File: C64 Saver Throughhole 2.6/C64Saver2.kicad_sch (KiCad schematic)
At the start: 24 parts, among them J1 Conn_01x04, J2 Conn_01x08, J4 Conn_01x08, J5 Conn_01x04, J6 Conn_01x04, Q1 BC547, Q2 IRFR5305, U1 TL431LP

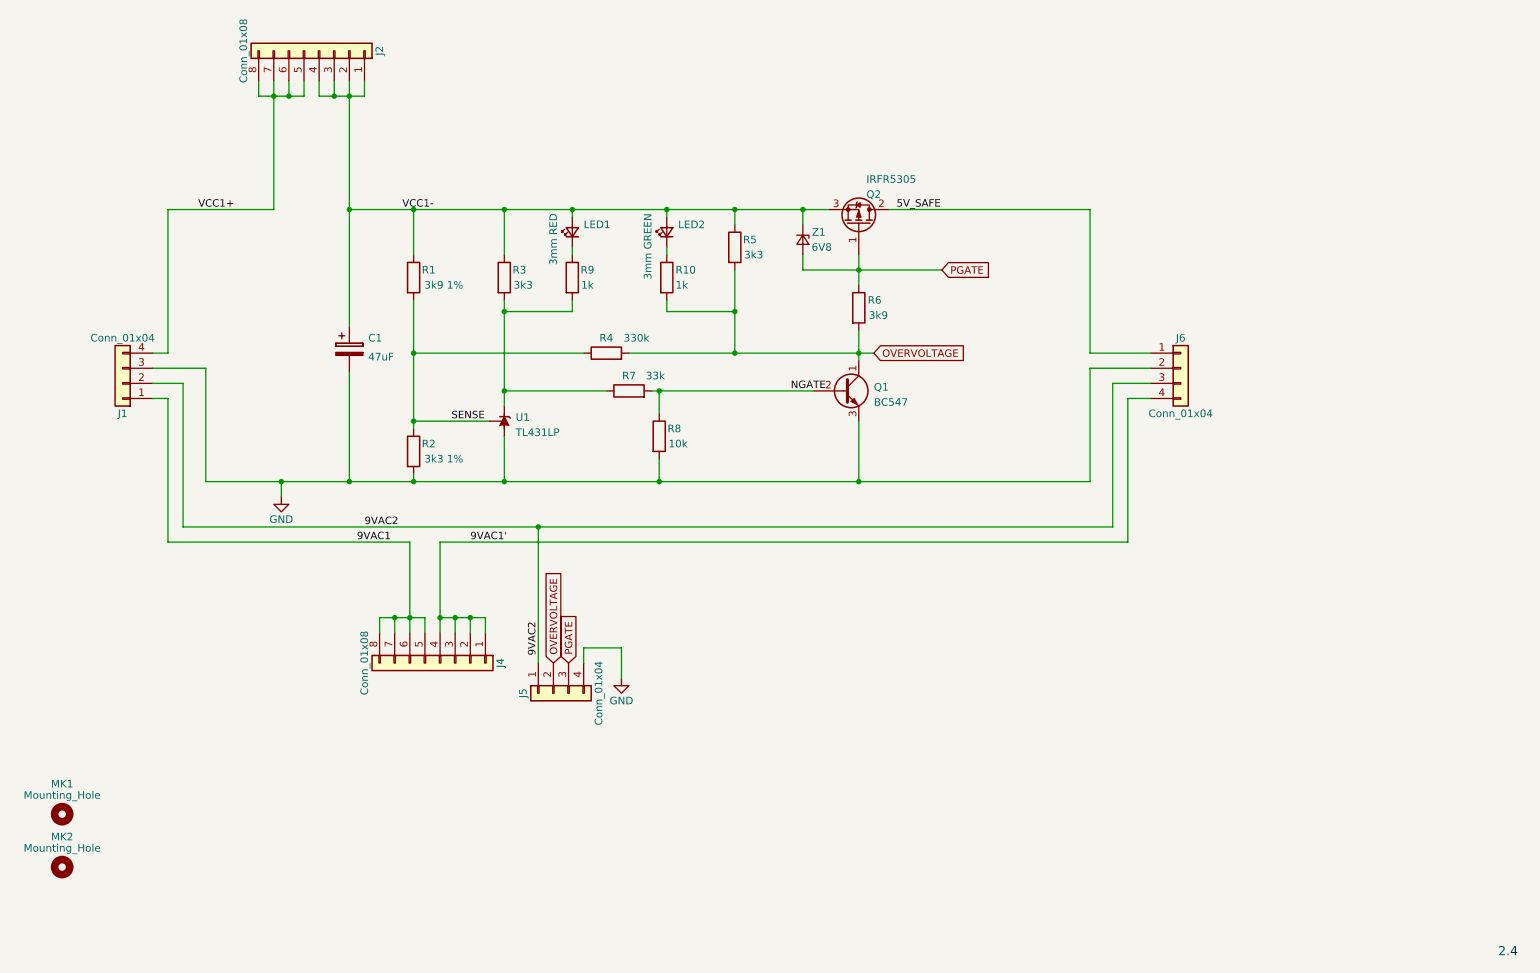
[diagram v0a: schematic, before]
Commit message: Preparing for Saver 2.6, moving 2.5 and 2.4 to oldfiles folder
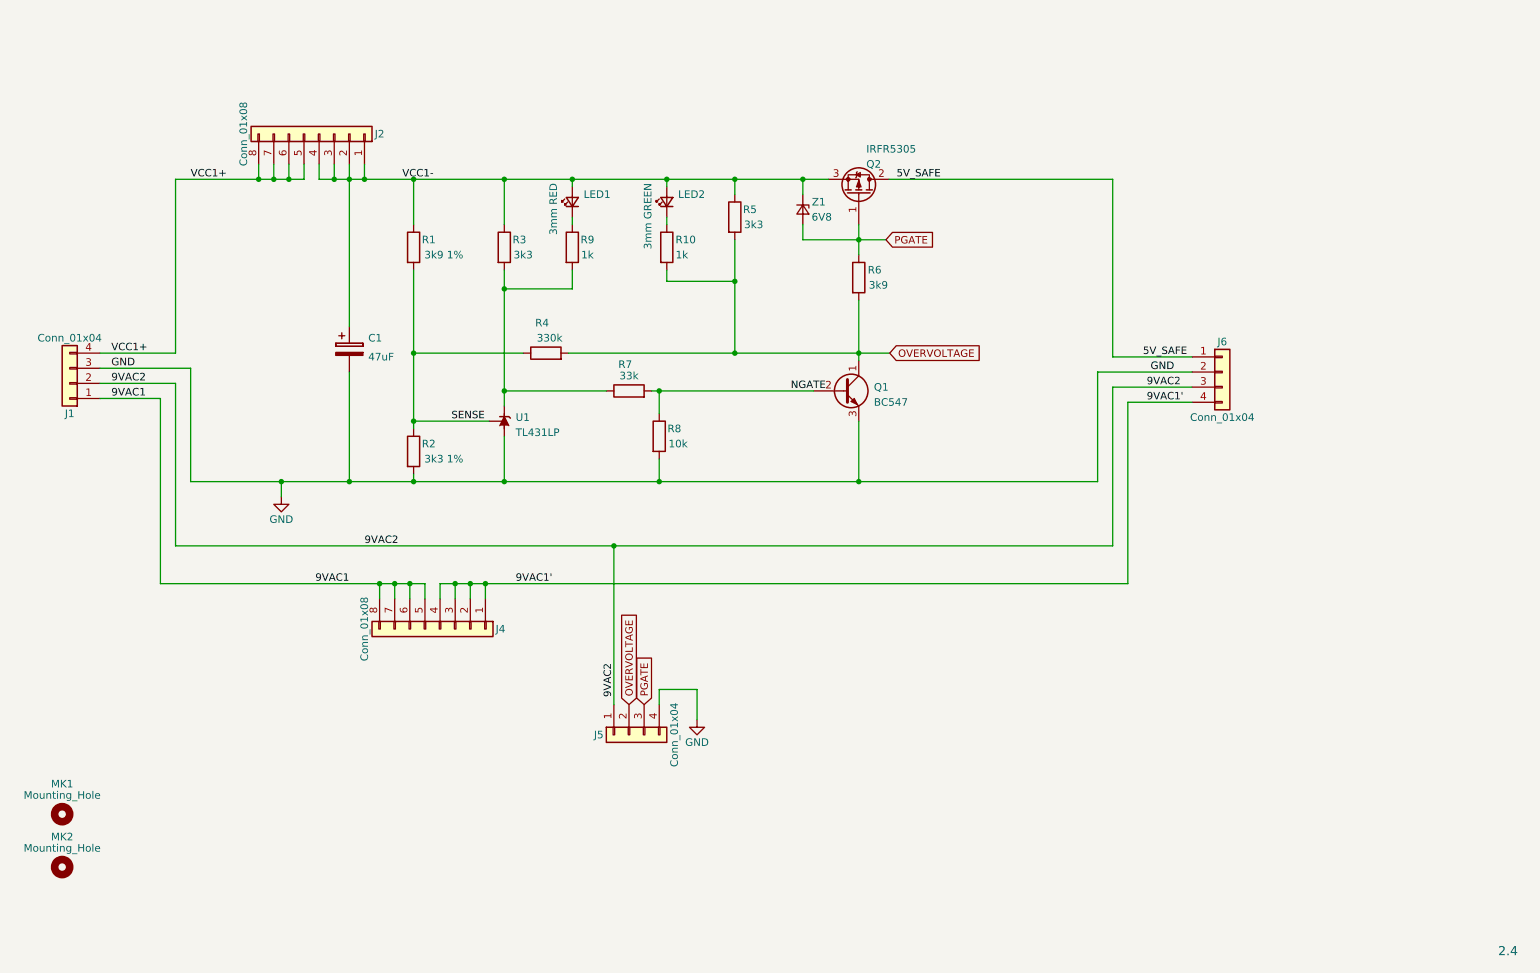
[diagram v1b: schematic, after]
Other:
- moved on the sheet: J1, J2, J4, J5, J6, LED1, LED2, Q2, R1, R10, R3, R4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
